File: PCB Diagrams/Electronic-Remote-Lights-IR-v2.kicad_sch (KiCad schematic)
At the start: 18 parts, among them J1 POWER, J2 220V, K1 RELAY, Q1 BC547, SW1 RESET, U1 VS1838B

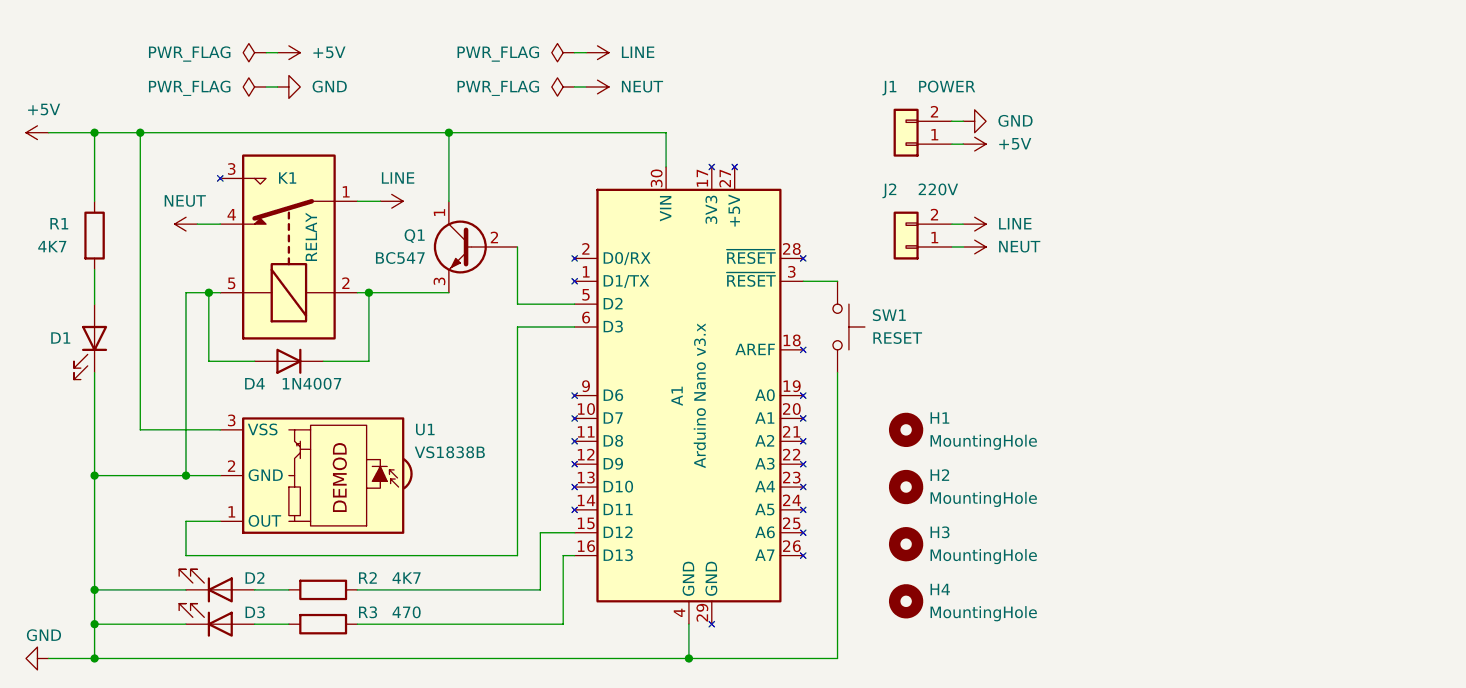
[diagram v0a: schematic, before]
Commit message: update track width to 1.5mm
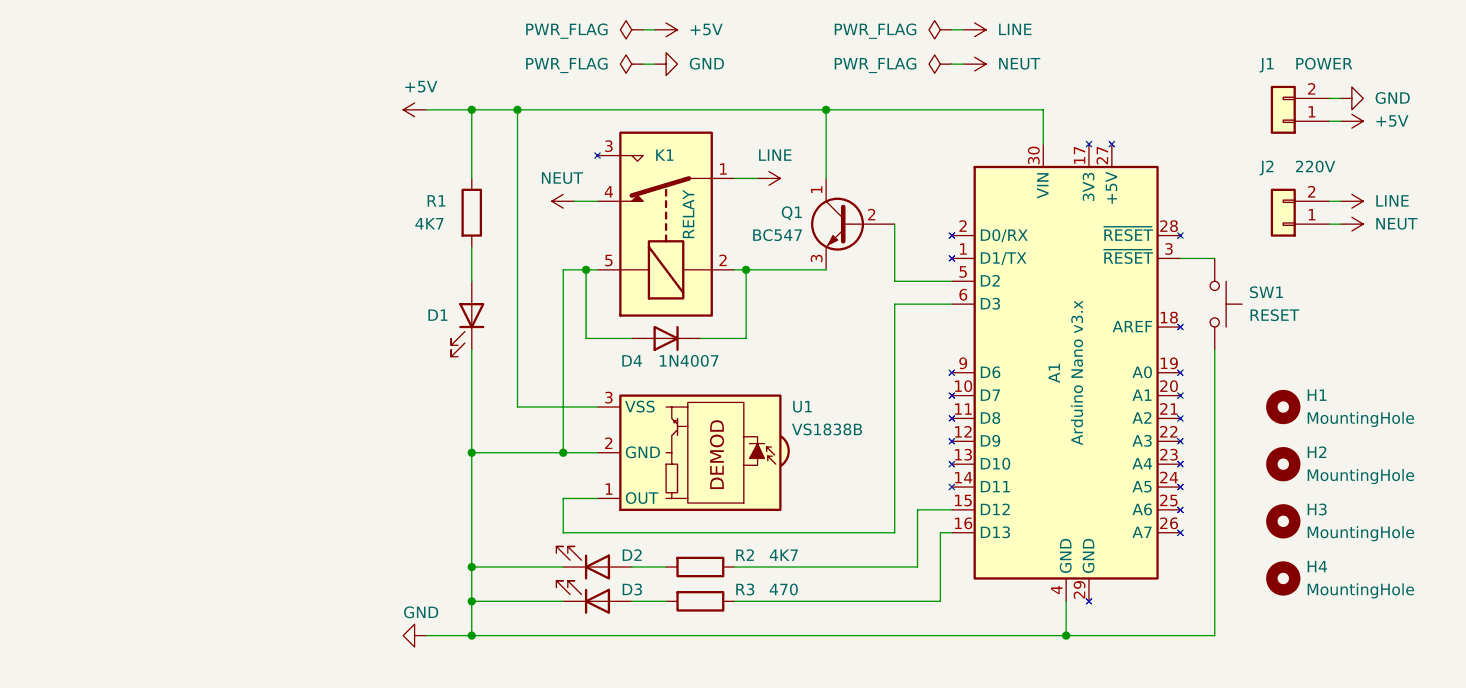
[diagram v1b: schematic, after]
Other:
- moved on the sheet: A1, D1, D2, D3, D4, H1, H2, H3, H4, J1, J2, K1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
